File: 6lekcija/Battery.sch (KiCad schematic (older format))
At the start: 2 parts

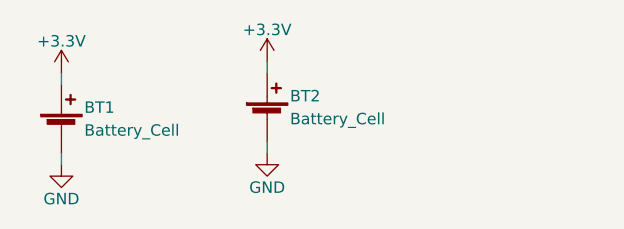
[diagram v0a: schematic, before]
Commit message: 6Lekcijas darba pabeigshana
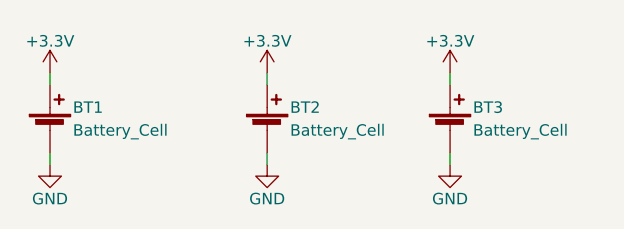
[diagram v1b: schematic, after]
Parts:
- added BT3: Battery_Cell, Battery_Holders:SMTU1225-LF, symbol Battery_Cell
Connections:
- net +3V3: now also BT3.1 (+)
- net GND: now also BT3.2 (-)
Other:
- moved on the sheet: BT1, BT2
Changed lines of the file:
@@
 L Battery_Cell BT1
 U 1 1 592692E8
-P 4450 2450
-F 0 "BT1" H 4550 2550 50  0000 L CNN
-F 1 "Battery_Cell" H 4550 2450 50  0000 L CNN
-F 2 "Battery_Holders:SMTU2032" V 4450 2510 50  0001 C CNN
-F 3 "" V 4450 2510 50  0001 C CNN
-	1    4450 2450
+P 4400 2450
+F 0 "BT1" H 4500 2550 50  0000 L CNN
+F 1 "Battery_Cell" H 4500 2450 50  0000 L CNN
+F 2 "Battery_Holders:SMTU2032" V 4400 2510 50  0001 C CNN
+F 3 "http://www.mouser.com/ds/2/346/SMTU2032-LF-6066.pdf" V 4400 2510 50  0001 C CNN
+	1    4400 2450
 	1    0    0    -1
 $EndComp
@@
 L +3.3V #PWR1
 U 1 1 592696CE
-P 4450 2200
-F 0 "#PWR1" H 4450 2050 50  0001 C CNN
-F 1 "+3.3V" H 4450 2340 50  0000 C CNN
-F 2 "" H 4450 2200 50  0001 C CNN
-F 3 "" H 4450 2200 50  0001 C CNN
-	1    4450 2200
+P 4400 2200
+F 0 "#PWR1" H 4400 2050 50  0001 C CNN
+F 1 "+3.3V" H 4400 2340 50  0000 C CNN
+F 2 "" H 4400 2200 50  0001 C CNN
+F 3 "" H 4400 2200 50  0001 C CNN
+	1    4400 2200
 	1    0    0    -1
 $EndComp
@@
 L GND #PWR2
 U 1 1 59269701
-P 4450 2600
-F 0 "#PWR2" H 4450 2350 50  0001 C CNN
-F 1 "GND" H 4450 2450 50  0000 C CNN
-F 2 "" H 4450 2600 50  0001 C CNN
-F 3 "" H 4450 2600 50  0001 C CNN
-	1    4450 2600
+P 4400 2600
+F 0 "#PWR2" H 4400 2350 50  0001 C CNN
+F 1 "GND" H 4400 2450 50  0000 C CNN
+F 2 "" H 4400 2600 50  0001 C CNN
+F 3 "" H 4400 2600 50  0001 C CNN
+	1    4400 2600
 	1    0    0    -1
 $EndComp
 Wire Wire Line
-	4450 2200 4450 2250
+	4400 2200 4400 2250
 Wire Wire Line
-	4450 2550 4450 2600
+	4400 2550 4400 2600
 $Comp
 L Battery_Cell BT2
 U 1 1 5926BEA1
-P 5350 2400
-F 0 "BT2" H 5450 2500 50  0000 L CNN
-F 1 "Battery_Cell" H 5450 2400 50  0000 L CNN
-F 2 "Battery_Holders:S8211R" V 5350 2460 50  0001 C CNN
-F 3 "" V 5350 2460 50  0001 C CNN
-	1    5350 2400
+P 5350 2450
+F 0 "BT2" H 5450 2550 50  0000 L CNN
+F 1 "Battery_Cell" H 5450 2450 50  0000 L CNN
+F 2 "Battery_Holders:S8211R" V 5350 2510 50  0001 C CNN
+F 3 "http://www.mouser.com/ds/2/181/S8211R-350557.pdf" V 5350 2510 50  0001 C CNN
+	1    5350 2450
 	1    0    0    -1
 $EndComp
@@
 L +3.3V #PWR3
 U 1 1 5926BEA7
-P 5350 2150
-F 0 "#PWR3" H 5350 2000 50  0001 C CNN
-F 1 "+3.3V" H 5350 2290 50  0000 C CNN
-F 2 "" H 5350 2150 50  0001 C CNN
-F 3 "" H 5350 2150 50  0001 C CNN
-	1    5350 2150
+P 5350 2200
+F 0 "#PWR3" H 5350 2050 50  0001 C CNN
+F 1 "+3.3V" H 5350 2340 50  0000 C CNN
+F 2 "" H 5350 2200 50  0001 C CNN
+F 3 "" H 5350 2200 50  0001 C CNN
+	1    5350 2200
 	1    0    0    -1
 $EndComp
@@
 L GND #PWR4
 U 1 1 5926BEAD
-P 5350 2550
-F 0 "#PWR4" H 5350 2300 50  0001 C CNN
-F 1 "GND" H 5350 2400 50  0000 C CNN
-F 2 "" H 5350 2550 50  0001 C CNN
-F 3 "" H 5350 2550 50  0001 C CNN
-	1    5350 2550
+P 5350 2600
+F 0 "#PWR4" H 5350 2350 50  0001 C CNN
+F 1 "GND" H 5350 2450 50  0000 C CNN
+F 2 "" H 5350 2600 50  0001 C CNN
+F 3 "" H 5350 2600 50  0001 C CNN
+	1    5350 2600
 	1    0    0    -1
 $EndComp
 Wire Wire Line
-	5350 2150 5350 2200
+	5350 2200 5350 2250
 Wire Wire Line
-	5350 2500 5350 2550
+	5350 2550 5350 2600
+$Comp
+L Battery_Cell BT3
+U 1 1 59427AC4
+P 6150 2450
+F 0 "BT3" H 6250 2550 50  0000 L CNN
+F 1 "Battery_Cell" H 6250 2450 50  0000 L CNN
+F 2 "Battery_Holders:SMTU1225-LF" V 6150 2510 50  0001 C CNN
+F 3 "http://www.mouser.com/ds/2/346/SMTU1225-LF-14436.pdf" V 6150 2510 50  0001 C CNN
+	1    6150 2450
+	1    0    0    -1
+$EndComp
+$Comp
+L GND #PWR?
+U 1 1 59427AEF
+P 6150 2600
+F 0 "#PWR?" H 6150 2350 50  0001 C CNN
+F 1 "GND" H 6150 2450 50  0000 C CNN
+F 2 "" H 6150 2600 50  0001 C CNN
+F 3 "" H 6150 2600 50  0001 C CNN
+	1    6150 2600
+	1    0    0    -1
+$EndComp
+$Comp
+L +3.3V #PWR?
+U 1 1 59427B03
+P 6150 2200
+F 0 "#PWR?" H 6150 2050 50  0001 C CNN
+F 1 "+3.3V" H 6150 2340 50  0000 C CNN
+F 2 "" H 6150 2200 50  0001 C CNN
+F 3 "" H 6150 2200 50  0001 C CNN
+	1    6150 2200
+	1    0    0    -1
+$EndComp
+Wire Wire Line
+	6150 2200 6150 2250
+Wire Wire Line
+	6150 2550 6150 2600
 $EndSCHEMATC
